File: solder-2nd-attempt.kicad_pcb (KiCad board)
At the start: 2 copper layers, 99.1 x 96.5 mm, 19 parts, among them Q1 NPN, Q2 NPN, Q3 NPN, SW1 SW_Push

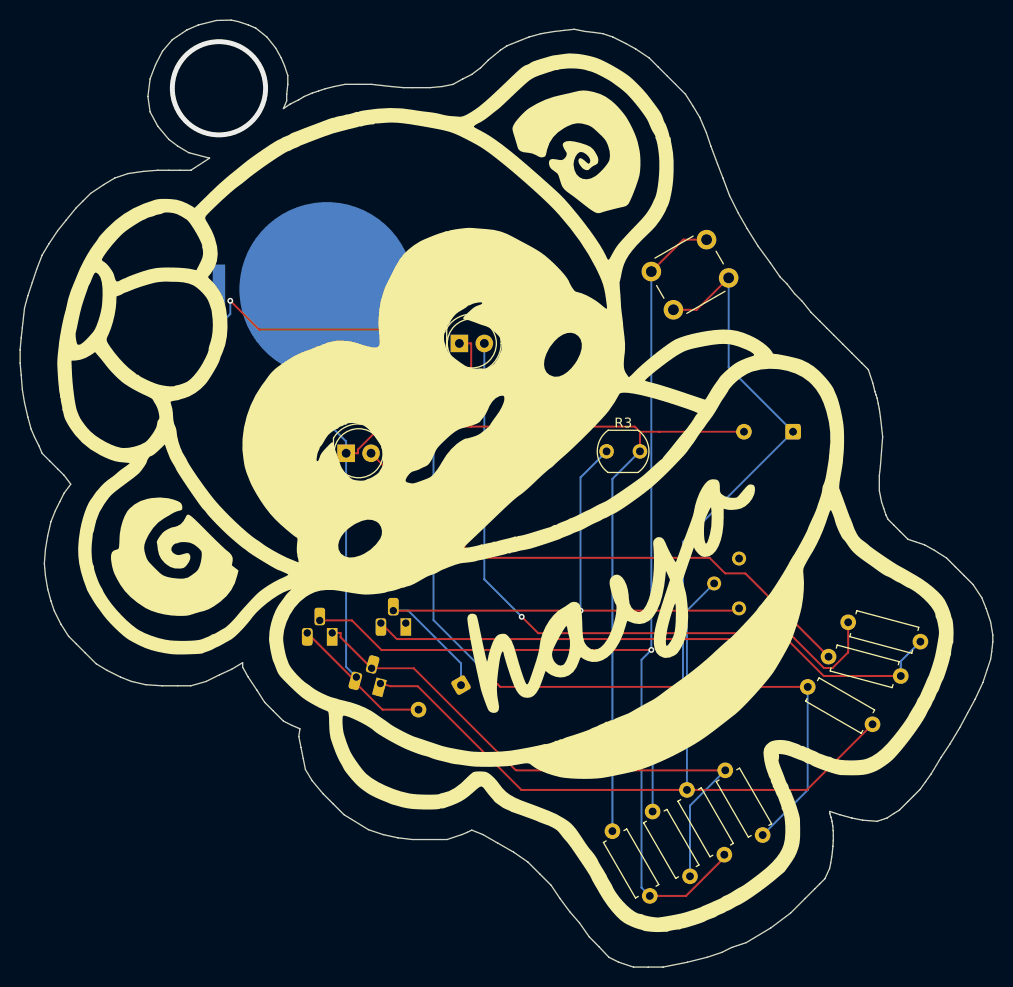
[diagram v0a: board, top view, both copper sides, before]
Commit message: updated schematic + pcb
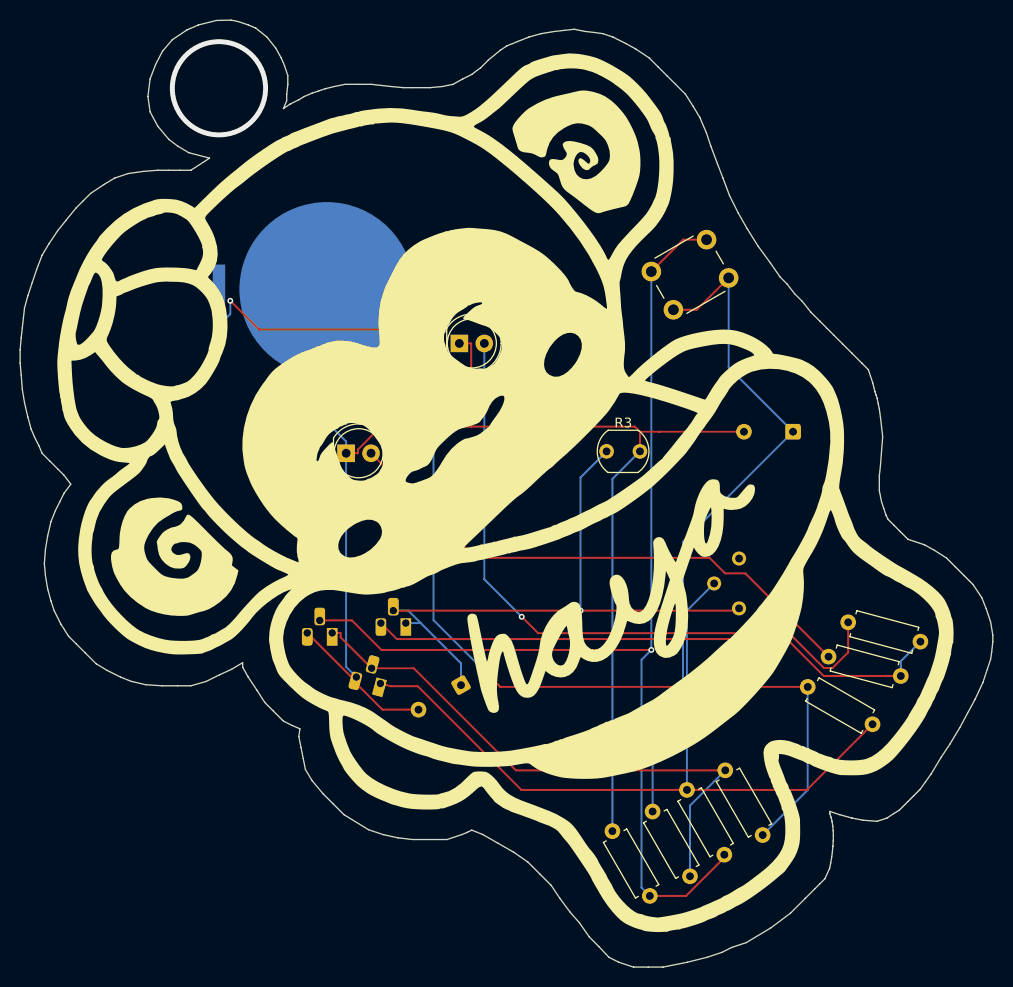
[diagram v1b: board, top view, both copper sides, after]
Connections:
- Q1 pad 1: unconnected-(Q1-C-Pad1) -> Net-(Q1-B)
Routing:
- net Net-(Q1-B): track 64.0 -> 65.5 mm
